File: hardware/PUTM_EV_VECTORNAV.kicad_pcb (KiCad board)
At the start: 4 copper layers, 70 x 70 mm, 91 parts, among them J1 Conn_01x02, J2 uFL ant, J3 SMA ant, J4 uFL ant, J5 SMA ant, J6 Conn_01x02, J7 USB_A, J8 FTSH-107-01-L-D-K, J9 XIAO ESP32S3 Sense, Q1 NMOS, Q2 SI2347DS-T1-GE3, U1 VN-300, U2 STM32G0C1KCTxN, U3 ADM3057ExRW, U4 FT231XS-U, U5 API7721FSB-13, U6 AQY284S, U7 NCP565D2T33R4G, U8 SI06W8-05

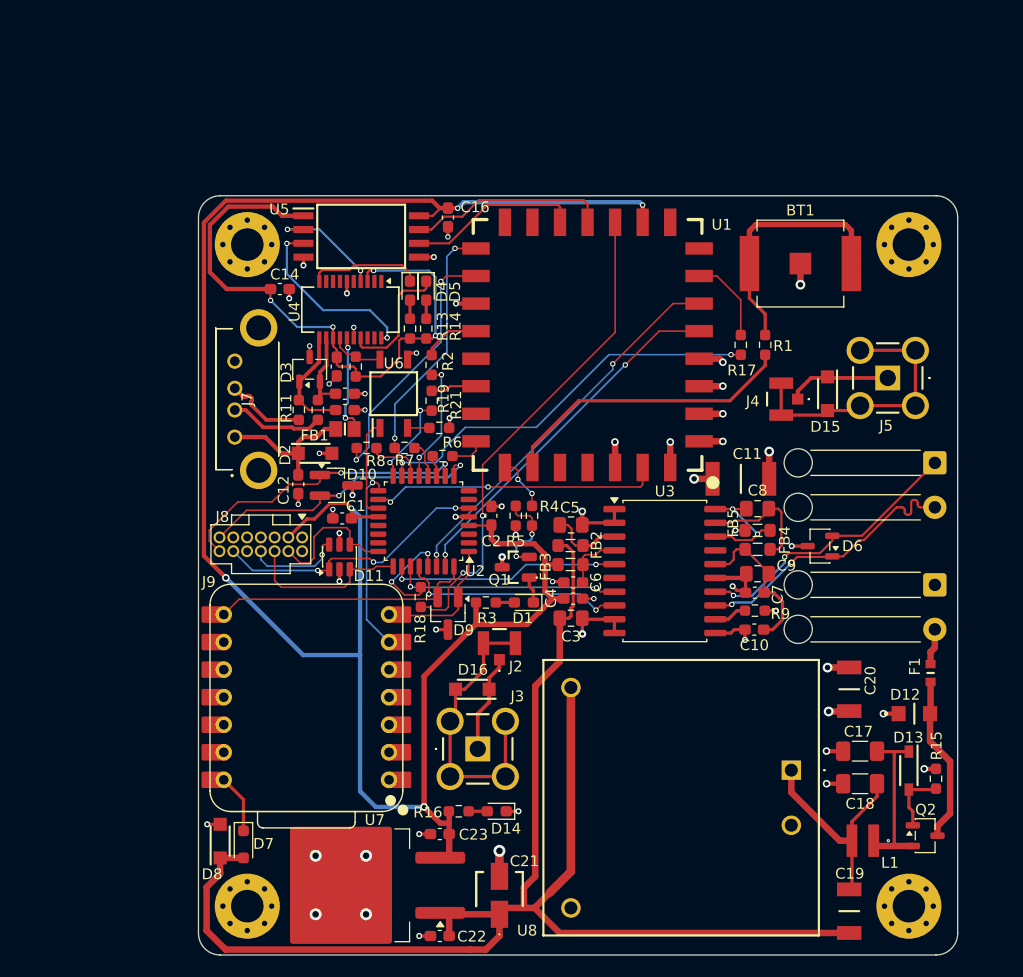
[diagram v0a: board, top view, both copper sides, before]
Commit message: Finished routing
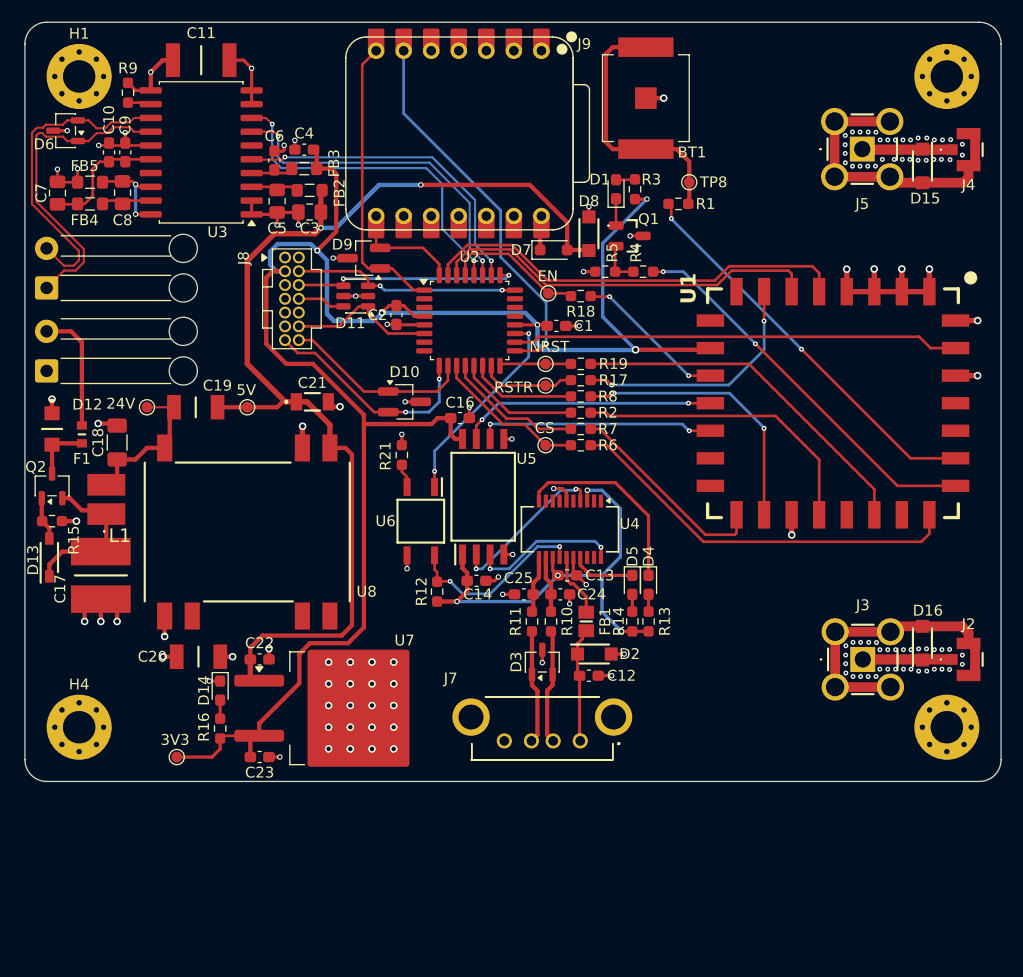
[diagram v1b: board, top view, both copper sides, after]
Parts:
- removed REF** (x4): MountingHole_3mm_Pad_Via, MountingHole:MountingHole_3mm_Pad_Via
- added H1: MountingHole_Pad, MountingHole:MountingHole_3mm_Pad_Via, F.Cu at (105.0, 35.0)
- added H2: MountingHole_Pad, MountingHole:MountingHole_3mm_Pad_Via, F.Cu at (185.0, 35.0)
- added H3: MountingHole_Pad, MountingHole:MountingHole_3mm_Pad_Via, F.Cu at (185.0, 95.0)
- added H4: MountingHole_Pad, MountingHole:MountingHole_3mm_Pad_Via, F.Cu at (105.0, 95.0)
- added TP1: 24V_TestPoint, TestPoint:TestPoint_Pad_D1.0mm, F.Cu at (111.2, 65.5)
- added TP2: 5V_TestPoint, TestPoint:TestPoint_Pad_D1.0mm, F.Cu at (120.5, 65.5)
- added TP3: 3V3_TestPoint, TestPoint:TestPoint_Pad_D1.0mm, F.Cu at (114.0, 97.8)
- added TP4: RSTR, TestPoint:TestPoint_Pad_D1.0mm, F.Cu at (148.0, 63.5)
- added TP5: NRST, TestPoint:TestPoint_Pad_D1.0mm, F.Cu at (148.0, 61.5)
- added TP6: EN, TestPoint:TestPoint_Pad_D1.0mm, F.Cu at (148.2, 55.0)
- added TP7: CS, TestPoint:TestPoint_Pad_D1.0mm, F.Cu at (148.0, 69.0)
- added TP8: BAT, TestPoint:TestPoint_Pad_D1.0mm, F.Cu at (161.2, 44.8)
- C17: value 2.2uF -> 10uF; footprint Capacitor_SMD:C_1206_3216Metric_Pad1.33x1.80mm_HandSolder -> 10uF24Vcap:CAPC6050X550N
- C21: value 47uF+ -> 20uF; footprint 47uCapPolarized:EEE1AA220WR -> 20uF5Vcap:GRM31x
- L1: value 10uH -> 3.9uH; footprint inductor:VLS3010 -> inductor:RLS397
- U8: value SI06W8-05 -> RSH3-2405S_H2; footprint DCisoconv:SI06W805 -> DCisoconv:RSH32405SH2
- moved Q2 86.7 mm to (102.5, 72.8), turned to 90 degrees
- moved R15 84.9 mm to (102.5, 76.0), turned to 180 degrees
- moved J6 84.2 mm to (102.0, 62.1), turned to 90 degrees
- moved D12 83.7 mm to (102.5, 67.5), turned to -90 degrees
- moved J1 83.5 mm to (102.0, 54.5), turned to 90 degrees
- moved D13 81.6 mm to (102.2, 79.3), turned to 90 degrees
- moved F1 81.3 mm to (105.2, 68.0)
- moved D6 79.4 mm to (103.8, 40.0)
- moved L1 76.5 mm to (107.5, 74.0), turned to 90 degrees
- moved C19 76.1 mm to (115.8, 65.5), turned to 0 degrees
- moved C18 75.4 mm to (108.5, 68.8), turned to 90 degrees
- moved R9 75.0 mm to (109.5, 36.5), turned to 90 degrees
- moved C7 73.5 mm to (103.0, 45.8), turned to -90 degrees
- moved C10 72.8 mm to (109.2, 42.0), turned to 90 degrees
- moved C9 72.1 mm to (107.8, 42.0), turned to -90 degrees
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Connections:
- D11 pad 3: /Connectors/PROG_SWCLK -> /Connectors/PROG_SWDIO
- D11 pad 4: /Connectors/PROG_SWDIO -> /Connectors/PROG_SWCLK
- D3 pad 1: /Connectors/d+ -> /Connectors/D+
- D3 pad 2: /Connectors/d- -> /Connectors/D-
- D6 pad 1: /CAN/CAN- -> /CAN/CAN+
- D6 pad 2: /CAN/CAN+ -> /CAN/CAN-
- U8 pad 1: Net-(U8-+VIN) -> GND_EXT
- U8 pad 2: GND_EXT -> unconnected-(U8-CTRL-Pad2)
- U8 pad 6: +5V -> unconnected-(U8-NC_1-Pad6)
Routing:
- net +5V: track 140.4 -> 103.1 mm, vias 0 -> 2
- net /MCU/VN_CS: track 3.25 -> 37.0 mm
- net Net-(U1-ENABLE): track 45.3 -> 14.1 mm
- net /VectorNav/GPS_PPS: track 5.10 -> 36.1 mm
- net Net-(U1-NRST): track 4.26 -> 33.3 mm
- net /MCU/VN_RESTORE: track 36.9 -> 8.87 mm, vias 2 -> 0
- net +3.3V: track 191.5 -> 167.5 mm
- net Net-(U1-SPI_MISO): track 5.37 -> 27.9 mm
- net /Connectors/XIAO_GPIO: track 17.1 -> 35.6 mm
- net /Connectors/XIAO_TX: track 11.6 -> 27.1 mm
- net Net-(U1-RESTORE): track 7.99 -> 22.9 mm, vias 0 -> 2
- net /Connectors/XIAO_RX: track 24.4 -> 9.67 mm
- net /MCU/VN_GNSS_SYNC: track 26.7 -> 41.3 mm, vias 2 -> 0
- net 3V3_USB: track 57.2 -> 43.0 mm
- net /MCU/vnCS: track 1.98 -> 14.2 mm
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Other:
- board size 70 x 70 mm -> 90 x 70 mm
- board text added: "24V"
- board text added: "3V3"
- board text added: "5V"
- board text added: "CS"
- board text added: "EN"
- board text added: "NRST"
- board text added: "RSTR"
- board text removed: "C4"
